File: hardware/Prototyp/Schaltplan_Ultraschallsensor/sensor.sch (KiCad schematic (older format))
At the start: 14 parts, among them U2 TLC272

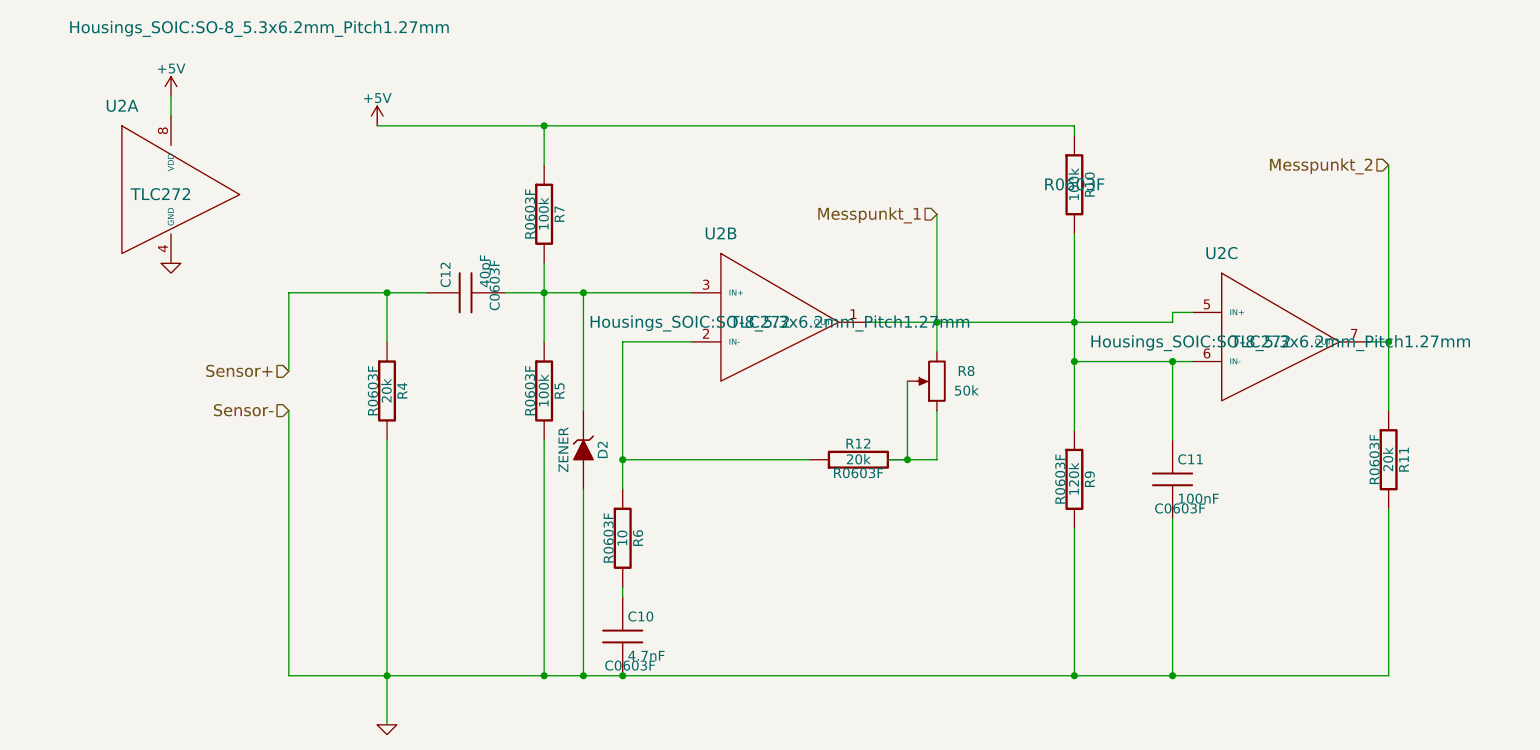
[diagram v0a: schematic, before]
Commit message: Schaltplanaktualisierung
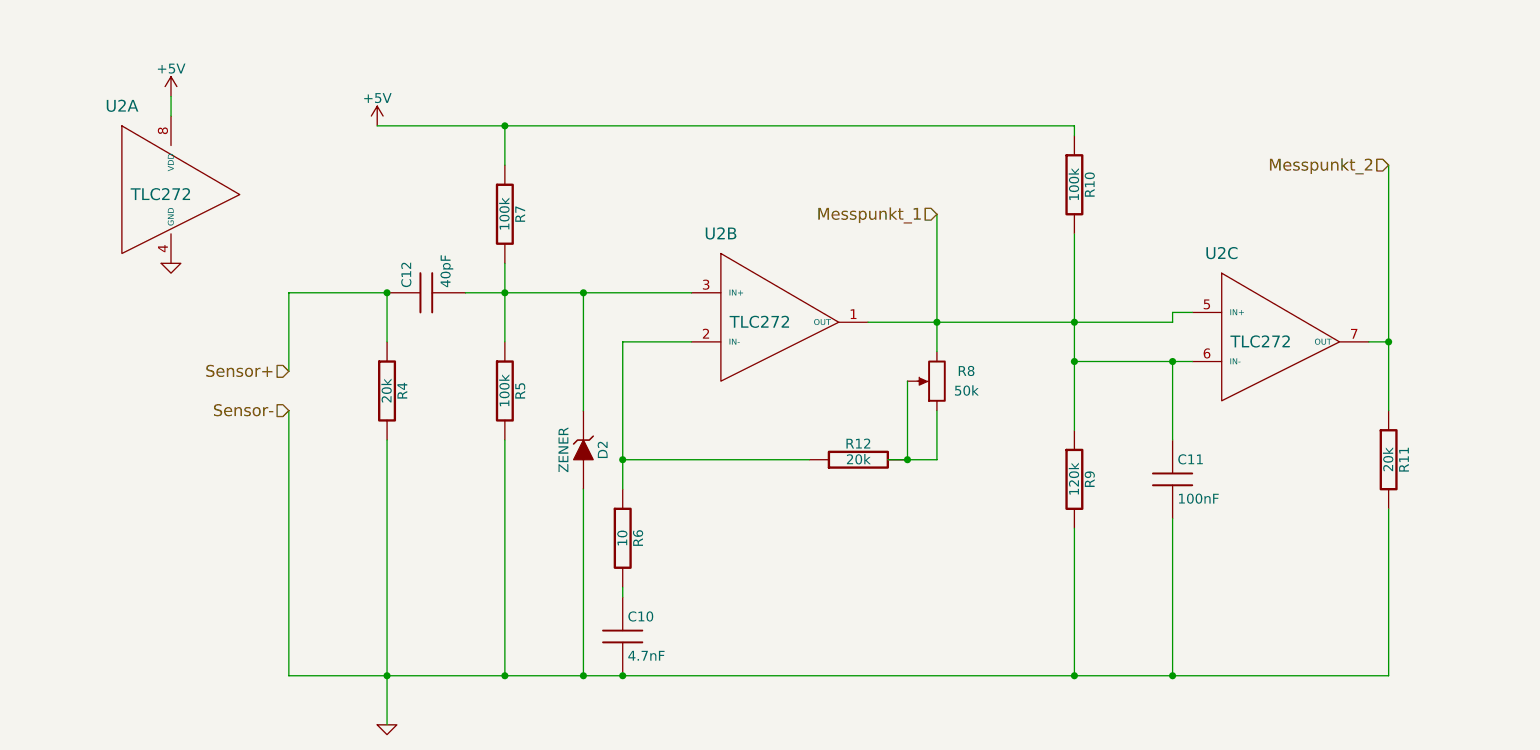
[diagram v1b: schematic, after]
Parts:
- C10, C11, C12: footprint C0603F -> kicad-libraries:C0603F
- D2: footprint (none) -> kicad-libraries:DO-214AA
- R10, R11, R12, R4, R5, R6, R7, R9: footprint R0603F -> kicad-libraries:R0603F
- R8: footprint (none) -> Zusatzteile:ST4ETA
- U2: footprint Housings_SOIC:SO-8_5.3x6.2mm_Pitch1.27mm -> kicad-libraries:TSSOP8
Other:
- moved on the sheet: C12, R5, R7
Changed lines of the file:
@@
 F 0 "R12" V 4680 2750 50  0000 C CNN
 F 1 "20k" V 4600 2750 50  0000 C CNN
-F 2 "R0603F" V 4530 2750 50  0000 C CNN
+F 2 "kicad-libraries:R0603F" V 4530 2750 50  0001 C CNN
 F 3 "" H 4600 2750 50  0000 C CNN
 	1    4600 2750
@@
 F 0 "R8" H 4850 2300 50  0000 C CNN
 F 1 "50k" H 4850 2400 50  0000 C CNN
-F 2 "" H 5000 2350 50  0000 C CNN
+F 2 "Zusatzteile:ST4ETA" H 5000 2350 50  0001 C CNN
 F 3 "" H 5000 2350 50  0000 C CNN
 	1    5000 2350
@@
 F 0 "R6" V 3480 3150 50  0000 C CNN
 F 1 "10" V 3400 3150 50  0000 C CNN
-F 2 "R0603F" V 3330 3150 50  0000 C CNN
+F 2 "kicad-libraries:R0603F" V 3330 3150 50  0001 C CNN
 F 3 "" H 3400 3150 50  0000 C CNN
 	1    3400 3150
@@
 F 0 "R9" V 5780 2850 50  0000 C CNN
 F 1 "120k" V 5700 2850 50  0000 C CNN
-F 2 "R0603F" V 5630 2850 50  0000 C CNN
+F 2 "kicad-libraries:R0603F" V 5630 2850 50  0001 C CNN
 F 3 "" H 5700 2850 50  0000 C CNN
 	1    5700 2850
@@
 L R R7
 U 1 1 5A4CED70
-P 3000 1500
-F 0 "R7" V 3080 1500 50  0000 C CNN
-F 1 "100k" V 3000 1500 50  0000 C CNN
-F 2 "R0603F" V 2930 1500 50  0000 C CNN
-F 3 "" H 3000 1500 50  0000 C CNN
-	1    3000 1500
+P 2800 1500
+F 0 "R7" V 2880 1500 50  0000 C CNN
+F 1 "100k" V 2800 1500 50  0000 C CNN
+F 2 "kicad-libraries:R0603F" V 2730 1500 50  0001 C CNN
+F 3 "" H 2800 1500 50  0000 C CNN
+	1    2800 1500
 	1    0    0    -1
 $EndComp
@@
 L R R5
 U 1 1 5A4CEDD5
-P 3000 2400
-F 0 "R5" V 3080 2400 50  0000 C CNN
-F 1 "100k" V 3000 2400 50  0000 C CNN
-F 2 "R0603F" V 2930 2400 50  0000 C CNN
-F 3 "" H 3000 2400 50  0000 C CNN
-	1    3000 2400
+P 2800 2400
+F 0 "R5" V 2880 2400 50  0000 C CNN
+F 1 "100k" V 2800 2400 50  0000 C CNN
+F 2 "kicad-libraries:R0603F" V 2730 2400 50  0001 C CNN
+F 3 "" H 2800 2400 50  0000 C CNN
+	1    2800 2400
 	1    0    0    -1
 $EndComp
@@
 F 0 "R4" V 2280 2400 50  0000 C CNN
 F 1 "20k" V 2200 2400 50  0000 C CNN
-F 2 "R0603F" V 2130 2400 50  0000 C CNN
+F 2 "kicad-libraries:R0603F" V 2130 2400 50  0001 C CNN
 F 3 "" H 2200 2400 50  0000 C CNN
 	1    2200 2400
@@
 L C C12
 U 1 1 5A4CEECB
-P 2600 1900
-F 0 "C12" H 2625 2000 50  0000 L CNN
-F 1 "40pF" H 2625 1800 50  0000 L CNN
-F 2 "C0603F" H 2638 1750 50  0000 C CNN
-F 3 "" H 2600 1900 50  0000 C CNN
-	1    2600 1900
+P 2400 1900
+F 0 "C12" H 2425 2000 50  0000 L CNN
+F 1 "40pF" H 2425 1800 50  0000 L CNN
+F 2 "kicad-libraries:C0603F" H 2438 1750 50  0001 C CNN
+F 3 "" H 2400 1900 50  0000 C CNN
+	1    2400 1900
 	0    -1   -1   0
 $EndComp
@@
 F 0 "C10" H 3425 3750 50  0000 L CNN
 F 1 "4.7nF" H 3425 3550 50  0000 L CNN
-F 2 "C0603F" H 3438 3500 50  0000 C CNN
+F 2 "kicad-libraries:C0603F" H 3438 3500 50  0001 C CNN
 F 3 "" H 3400 3650 50  0000 C CNN
 	1    3400 3650
@@
 F 0 "C11" H 6225 2950 50  0000 L CNN
 F 1 "100nF" H 6225 2750 50  0000 L CNN
-F 2 "C0603F" H 6238 2700 50  0000 C CNN
+F 2 "kicad-libraries:C0603F" H 6238 2700 50  0001 C CNN
 F 3 "" H 6200 2850 50  0000 C CNN
 	1    6200 2850
@@
 F 0 "R11" V 7380 2750 50  0000 C CNN
 F 1 "20k" V 7300 2750 50  0000 C CNN
-F 2 "R0603F" V 7230 2750 50  0000 C CNN
+F 2 "kicad-libraries:R0603F" V 7230 2750 50  0001 C CNN
 F 3 "" H 7300 2750 50  0000 C CNN
 	1    7300 2750
@@
 F 0 "R10" V 5780 1350 50  0000 C CNN
 F 1 "100k" V 5700 1350 50  0000 C CNN
-F 2 "R0603F" H 5700 1350 60  0000 C CNN
+F 2 "kicad-libraries:R0603F" H 5700 1350 60  0001 C CNN
 F 3 "" H 5700 1350 60  0000 C CNN
 	1    5700 1350
@@
 	3400 3400 3400 3450
 Wire Wire Line
-	1700 1900 2400 1900
-Wire Wire Line
 	2200 1900 2200 2150
 Connection ~ 2200 1900
-Connection ~ 3000 1900
-Wire Wire Line
-	3000 1050 3000 1250
 Wire Wire Line
 	2150 1050 5700 1050
-Connection ~ 3000 1050
 Wire Wire Line
 	3400 2150 3400 2900
@@
 Connection ~ 3400 2750
 Wire Wire Line
-	3000 1750 3000 2150
-Wire Wire Line
-	3000 3850 3000 2650
-Connection ~ 3000 3850
-Wire Wire Line
 	3400 2150 3750 2150
 Wire Wire Line
-	2800 1900 3750 1900
+	2600 1900 3750 1900
 Wire Wire Line
 	6200 2250 6200 2650
@@
 Connection ~ 5700 3850
 $Comp
-L GND #PWR021
+L GND #PWR027
 U 1 1 5A70B233
 P 2200 4100
-F 0 "#PWR021" H 2200 4100 30  0001 C CNN
+F 0 "#PWR027" H 2200 4100 30  0001 C CNN
 F 1 "GND" H 2200 4030 30  0001 C CNN
 F 2 "" H 2200 4100 60  0000 C CNN
@@
 $EndComp
 $Comp
-L +5V #PWR022
+L +5V #PWR028
 U 1 1 5A70745C
 P 2150 1050
-F 0 "#PWR022" H 2150 900 50  0001 C CNN
+F 0 "#PWR028" H 2150 900 50  0001 C CNN
 F 1 "+5V" H 2150 1190 50  0000 C CNN
 F 2 "" H 2150 1050 50  0001 C CNN
@@
 F 0 "U2" H 3900 2500 60  0000 C CNN
 F 1 "TLC272" H 4100 2050 60  0000 C CNN
-F 2 "Housings_SOIC:SO-8_5.3x6.2mm_Pitch1.27mm" H 4200 2050 60  0000 C CNN
+F 2 "kicad-libraries:TSSOP8" H 4200 2050 60  0001 C CNN
 F 3 "" H 4200 2050 60  0000 C CNN
 	2    4200 2050
@@
 F 0 "U2" H 6450 2600 60  0000 C CNN
 F 1 "TLC272" H 6650 2150 60  0000 C CNN
-F 2 "Housings_SOIC:SO-8_5.3x6.2mm_Pitch1.27mm" H 6750 2150 60  0000 C CNN
+F 2 "kicad-libraries:TSSOP8" H 6750 2150 60  0001 C CNN
 F 3 "" H 6750 2150 60  0000 C CNN
 	3    6750 2150
@@
 F 0 "U2" H 850 1850 60  0000 C CNN
 F 1 "TLC272" H 1050 1400 60  0000 C CNN
-F 2 "Housings_SOIC:SO-8_5.3x6.2mm_Pitch1.27mm" H 1550 2250 60  0000 C CNN
+F 2 "kicad-libraries:TSSOP8" H 1550 2250 60  0001 C CNN
 F 3 "" H 1150 1400 60  0000 C CNN
 	1    1150 1400
@@
 $EndComp
 $Comp
-L GND #PWR023
+L GND #PWR029
 U 1 1 5A711570
 P 1100 1750
-F 0 "#PWR023" H 1100 1750 30  0001 C CNN
+F 0 "#PWR029" H 1100 1750 30  0001 C CNN
 F 1 "GND" H 1100 1680 30  0001 C CNN
 F 2 "" H 1100 1750 60  0000 C CNN
@@
 $EndComp
 $Comp
-L +5V #PWR024
+L +5V #PWR030
 U 1 1 5A7115A2
 P 1100 900
-F 0 "#PWR024" H 1100 750 50  0001 C CNN
+F 0 "#PWR030" H 1100 750 50  0001 C CNN
 F 1 "+5V" H 1100 1040 50  0000 C CNN
 F 2 "" H 1100 900 50  0001 C CNN
@@
 F 0 "D2" H 3200 2800 50  0000 C CNN
 F 1 "ZENER" H 3200 2600 50  0000 C CNN
-F 2 "" H 3200 2700 50  0000 C CNN
+F 2 "kicad-libraries:DO-214AA" H 3200 2700 50  0001 C CNN
 F 3 "" H 3200 2700 50  0000 C CNN
 	1    3200 2700
@@
 	3200 2900 3200 3850
 Connection ~ 3200 3850
+Wire Wire Line
+	2800 1750 2800 2150
+Connection ~ 2800 1900
+Wire Wire Line
+	2200 1900 1700 1900
+Wire Wire Line
+	2800 1250 2800 1050
+Connection ~ 2800 1050
+Wire Wire Line
+	2800 2650 2800 3850
+Connection ~ 2800 3850
 $EndSCHEMATC
